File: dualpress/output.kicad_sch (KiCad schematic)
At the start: 25 parts, among them Q2 SS8050, Q3 SS8050, U1 LD1117S33TR_SOT223

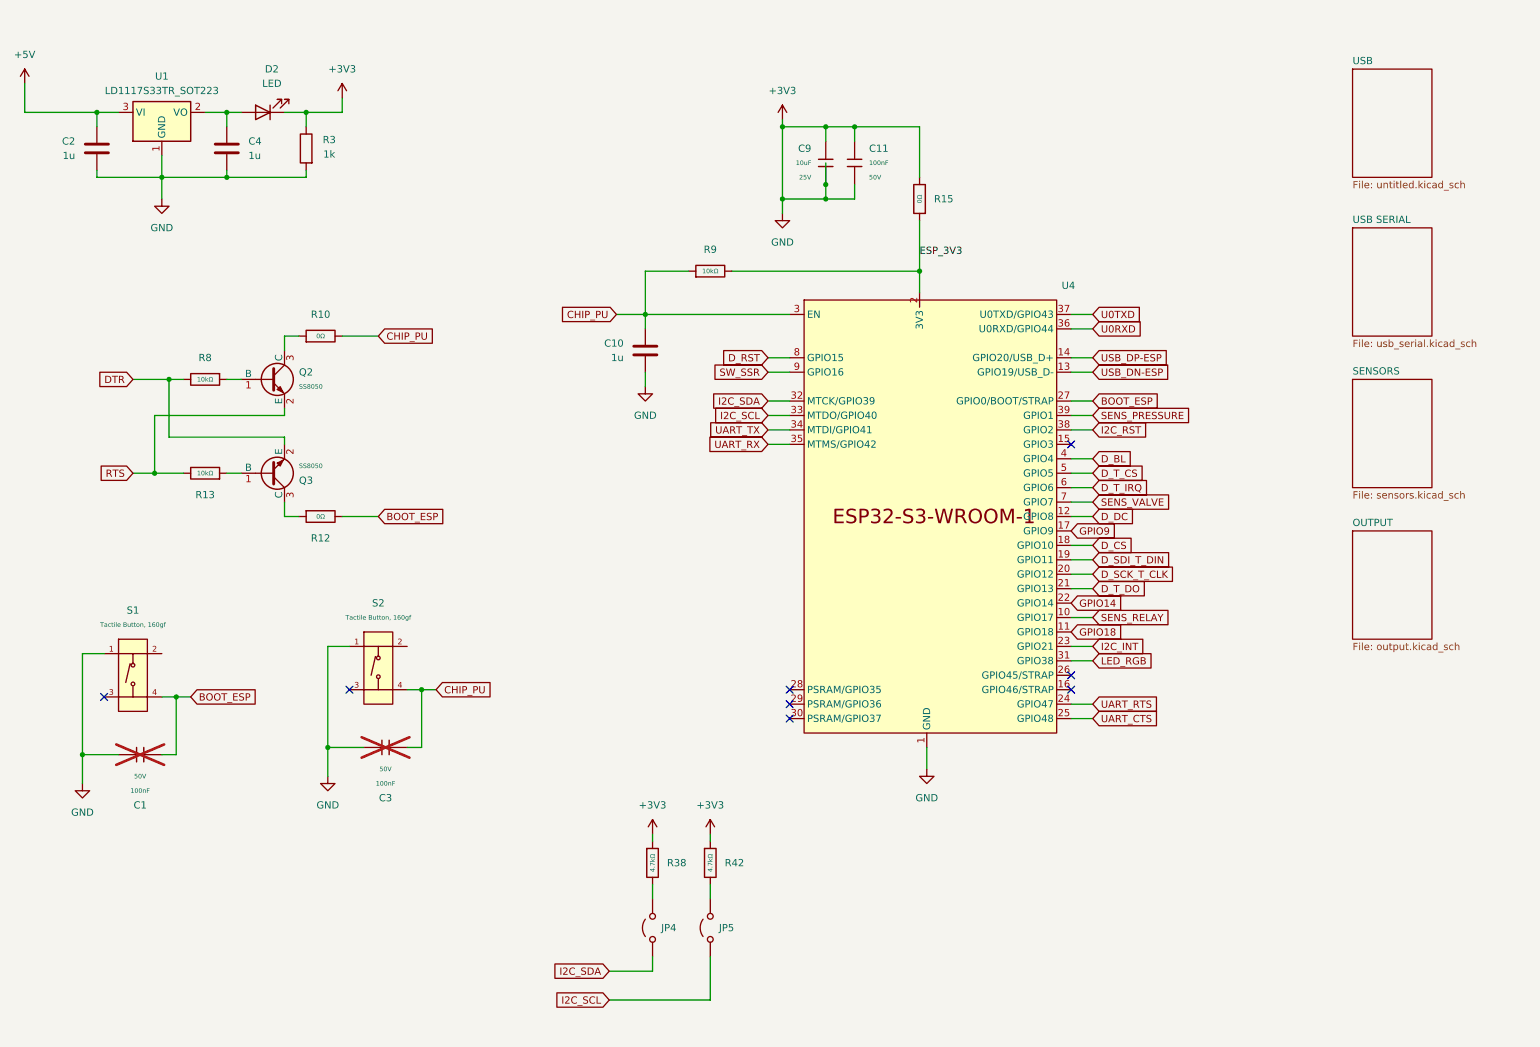
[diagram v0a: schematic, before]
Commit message: schematic done
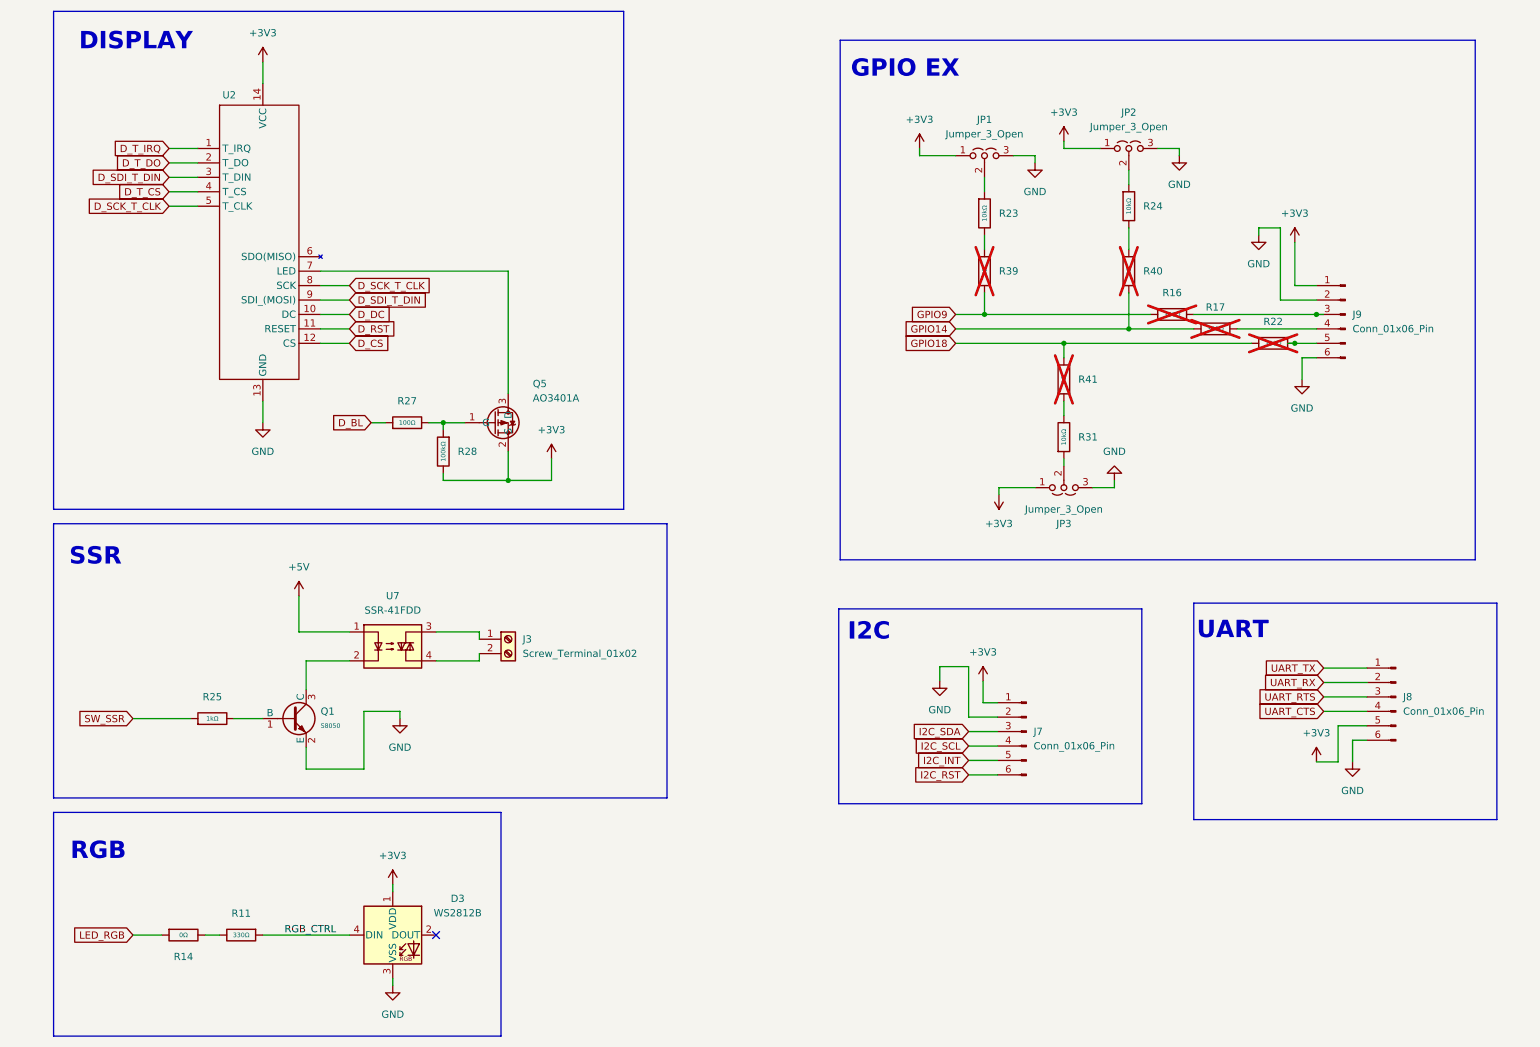
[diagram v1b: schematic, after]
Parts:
- removed C1, C11, C3: 100nF, PCM_JLCPCB:C_0603, symbol PCM_JLCPCB-Capacitors:0603,100nF
- removed C10, C2, C4: 1u, Capacitor_SMD:C_0805_2012Metric, symbol Device:C
- removed C9: 10uF, PCM_JLCPCB:C_0603, symbol PCM_JLCPCB-Capacitors:0603,10uF,(2)
- removed D2: LED, Diode_SMD:D_0201_0603Metric, symbol Device:LED
- removed JP4, JP5: Jumper_2_Open, symbol Jumper:Jumper_2_Open
- removed Q2, Q3: SS8050, PCM_JLCPCB:Q_SOT-23, symbol PCM_JLCPCB-Transistors:NPN,SS8050,(2)
- removed R10, R12, R15: 0Ω, PCM_JLCPCB:R_0603, symbol PCM_JLCPCB-Resistors:0603,0Ω
- removed R13, R8, R9: 10kΩ, PCM_JLCPCB:R_0603, symbol PCM_JLCPCB-Resistors:0603,10kΩ
- removed R3: 1k, Resistor_SMD:R_0805_2012Metric, symbol Device:R
- removed R38, R42: 4.7kΩ, PCM_JLCPCB:R_0603, symbol PCM_JLCPCB-Resistors:0603,4.7kΩ
- removed S1, S2: Tactile Button, 160gf, PCM_JLCPCB:SW-SMD_4P-L5.1-W5.1-P3.70-LS6.5-TL-2, symbol PCM_JLCPCB-Connectors_Buttons:Tactile Button, 160gf, 12V, 50mA, 5.1mm
- removed U1: LD1117S33TR_SOT223, Package_TO_SOT_SMD:SOT-223-3_TabPin2, symbol Regulator_Linear:LD1117S33TR_SOT223
- removed U4: (no value), symbol 01_dualpress:ESP32-S2-WROOM-1-N16R8
- added D3: WS2812B, PCM_JLCPCB:LED_WS2812B_PLCC4_5.0x5.0mm_P3.2mm, symbol PCM_JLCPCB-Extended:LED, WS2812B, 5050
- added J3: Screw_Terminal_01x02, symbol Connector:Screw_Terminal_01x02
- added J7, J8, J9: Conn_01x06_Pin, symbol Connector:Conn_01x06_Pin
- added JP1, JP2, JP3: Jumper_3_Open, symbol Jumper:Jumper_3_Open
- added Q1: S8050, PCM_JLCPCB:Q_SOT-23, symbol PCM_JLCPCB-Transistors:NPN,S8050
- added Q5: AO3401A, Package_TO_SOT_SMD:SOT-23, symbol Transistor_FET:AO3401A
- added R11: 330Ω, PCM_JLCPCB:R_0603, symbol PCM_JLCPCB-Resistors:0603,330Ω
- added R14, R39, R40, R41: 0Ω, PCM_JLCPCB:R_0603, symbol PCM_JLCPCB-Resistors:0603,0Ω
- added R16, R17, R22: 300Ω, PCM_JLCPCB:R_1206, symbol PCM_JLCPCB-Resistors:1206,300Ω
- added R23, R24, R31: 10kΩ, PCM_JLCPCB:R_0603, symbol PCM_JLCPCB-Resistors:0603,10kΩ
- added R25: 1kΩ, PCM_JLCPCB:R_0603, symbol PCM_JLCPCB-Resistors:0603,1kΩ
- added R27: 100Ω, PCM_JLCPCB:R_0805, symbol PCM_JLCPCB-Resistors:0805,100Ω
- added R28: 100kΩ, PCM_JLCPCB:R_0805, symbol PCM_JLCPCB-Resistors:0805,100kΩ
- added U2: 2.8" Touch Display SPI 14x1, symbol 01_dualpress:2.8{dblquote} Touch Display SPI 14x1
- added U7: SSR-41FDD, 01_dualpress:SSR-41FDD, symbol 01_dualpress:SSR-41FDD
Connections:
- net +3V3: now also D3.1 (VDD), J7.1 (Pin_1), J8.5 (Pin_5), J9.1 (Pin_1), JP1.1 (A), JP2.1 (A), JP3.1 (A), Q5.2 (S), R28.2, U2.14 (VCC)
- net +5V: now also U7.1
- net D_BL: now also R27.1
- net D_CS: now also U2.12 (CS)
- net D_DC: now also U2.10 (DC)
- net D_RST: now also U2.11 (RESET)
- net D_SCK_T_CLK: now also U2.5 (T_CLK), U2.8 (SCK)
- net D_SDI_T_DIN: now also U2.3 (T_DIN), U2.9 (SDI_(MOSI))
- net D_T_CS: now also U2.4 (T_CS)
- net D_T_DO: now also U2.2 (T_DO)
- net D_T_IRQ: now also U2.1 (T_IRQ)
- net GPIO14: now also R17.1, R40.2
- net GPIO18: now also R22.1, R41.1
- net GPIO9: now also R16.1, R39.2
- net I2C_INT: now also J7.5 (Pin_5)
- net I2C_RST: now also J7.6 (Pin_6)
- net I2C_SCL: now also J7.4 (Pin_4)
- net I2C_SDA: now also J7.3 (Pin_3)
- net LED_RGB: now also R14.1
- net SW_SSR: now also R25.1
- net UART_CTS: now also J8.4 (Pin_4)
- net UART_RTS: now also J8.3 (Pin_3)
- net UART_RX: now also J8.2 (Pin_2)
- net UART_TX: now also J8.1 (Pin_1)
- new net: Q1.3 (C), U7.2
- new net: J3.1 (Pin_1), U7.3
- new net: J3.2 (Pin_2), U7.4
- new net: R11.2, R14.2
- new net: Q1.1 (B), R25.2
- new net: JP3.2 (C), R31.1
- new net: R31.2, R41.2
- new net: R23.2, R39.1
- new net: Q5.1 (G), R27.2, R28.1
- new net: JP1.2 (C), R23.1
- new net: J9.5 (Pin_5), R22.2
- new net: JP2.2 (C), R24.1
- new net: R24.2, R40.1
- new net: J9.3 (Pin_3), R16.2
- new net: J9.4 (Pin_4), R17.2
- new net: Q5.3 (D), U2.7 (LED)
- new net GND: D3.3 (VSS), J7.2 (Pin_2), J8.6 (Pin_6), J9.2 (Pin_2), J9.6 (Pin_6), JP1.3 (B), JP2.3 (B), JP3.3 (B), Q1.2 (E), U2.13 (GND)
- new net RGB_CTRL: D3.4 (DIN), R11.1
- no-connect marks 8 -> 1
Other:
- removed sheet OUTPUT
- removed sheet SENSORS
- removed sheet USB
- removed sheet USB SERIAL
- note added: "DISPLAY"
- note added: "GPIO EX"
- note added: "I2C"
- note added: "RGB"
- note added: "SSR"
- note added: "UART"
